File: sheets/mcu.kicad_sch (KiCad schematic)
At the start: 10 parts, among them U1 STM32F072CBTx

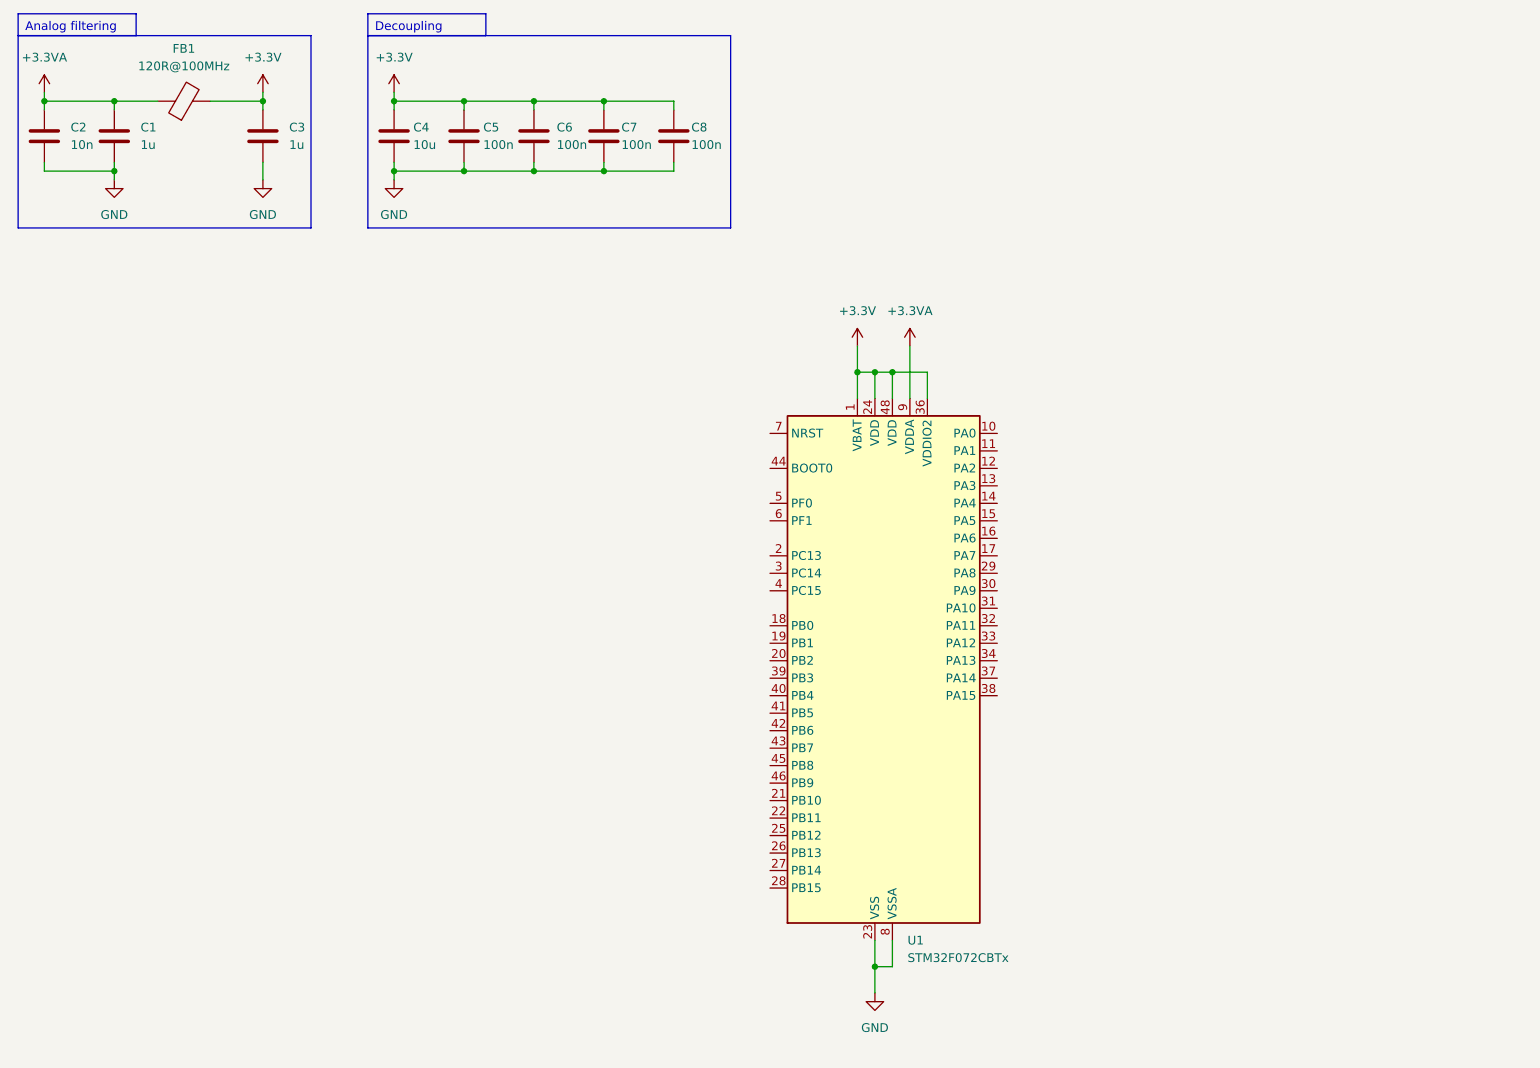
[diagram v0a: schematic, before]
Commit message: fsdfsdf
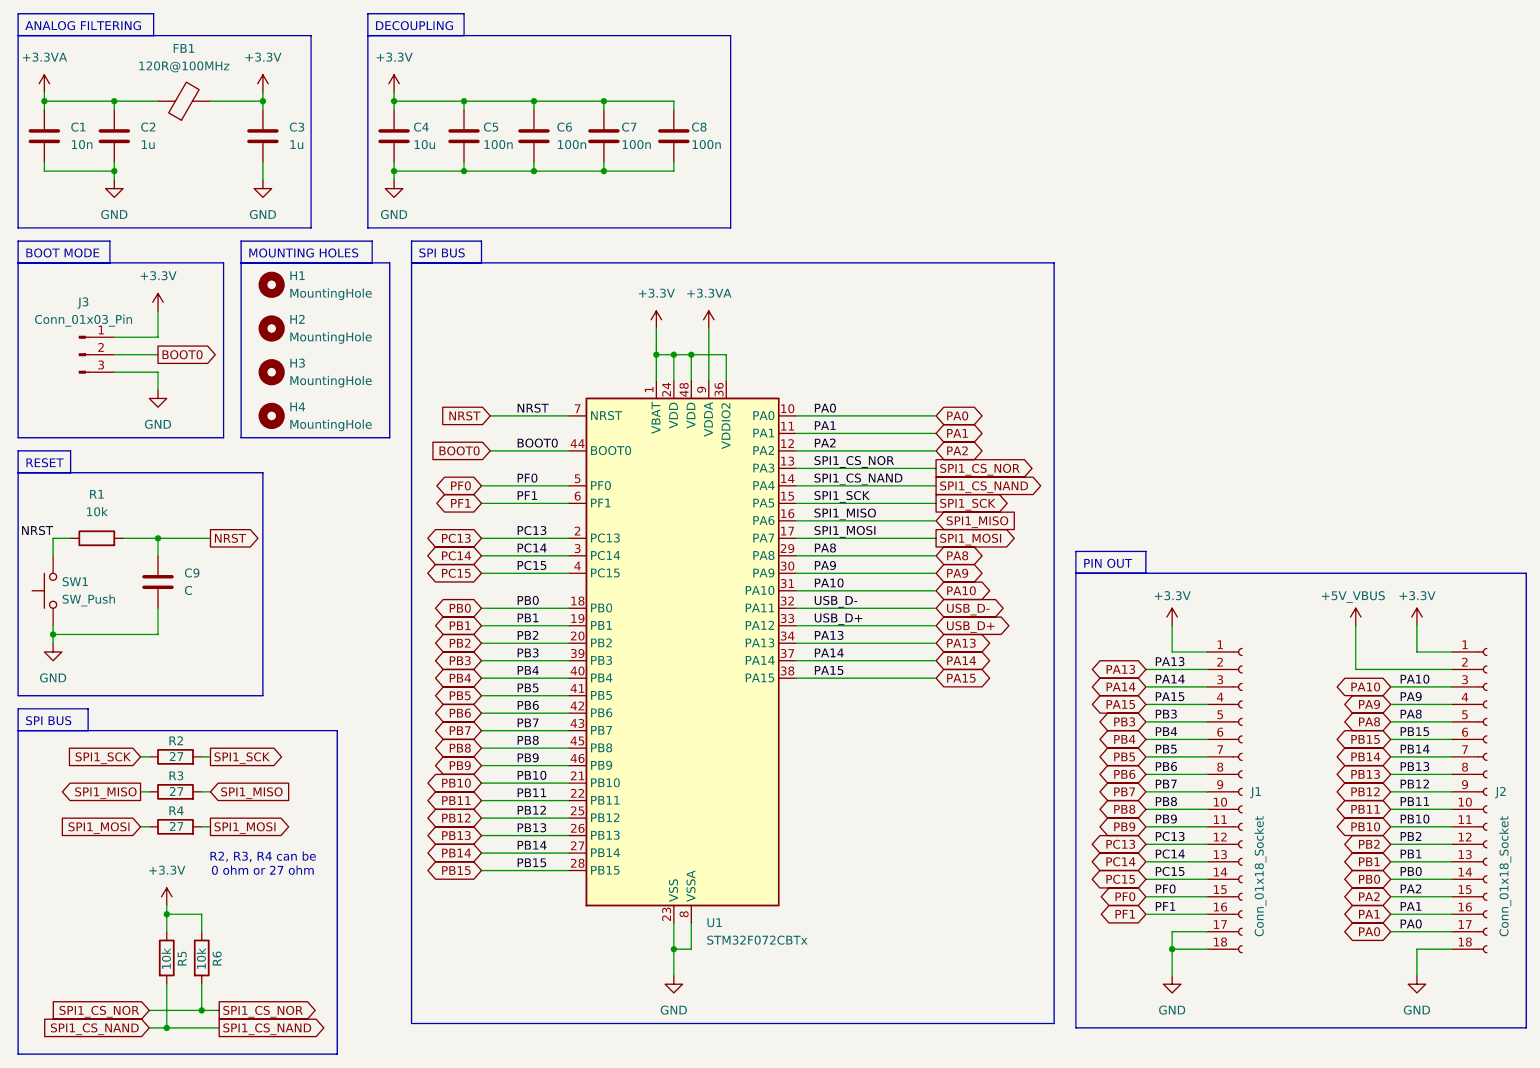
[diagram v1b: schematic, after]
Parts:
- added C9: C, Capacitor_SMD:C_0603_1608Metric, symbol Device:C
- added H1, H2, H3, H4: MountingHole, MountingHole:MountingHole_2.2mm_M2_DIN965, symbol Mechanical:MountingHole
- added J1, J2: Conn_01x18_Socket, Connector_PinSocket_2.54mm:PinSocket_1x18_P2.54mm_Vertical, symbol Connector:Conn_01x18_Socket
- added J3: Conn_01x03_Pin, Connector_PinHeader_2.54mm:PinHeader_1x03_P2.54mm_Vertical, symbol Connector:Conn_01x03_Pin
- added R1, R5, R6: 10k, Resistor_SMD:R_0603_1608Metric, symbol Device:R
- added R2, R3, R4: 27, Resistor_SMD:R_0603_1608Metric, symbol Device:R
- added SW1: SW_Push, Button_Switch_SMD:SW_Push_SPST_NO_Alps_SKRK, symbol Switch:SW_Push
- FB1: footprint (none) -> Resistor_SMD:R_0603_1608Metric
- renumbered C2 to C1, C1 to C2
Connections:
- net +3.3V: now also J1.1 (Pin_1), J2.1 (Pin_1), J3.1 (Pin_1), R5.1, R6.1
- net GND: now also C9.2, J1.17 (Pin_17), J1.18 (Pin_18), J2.18 (Pin_18), J3.3 (Pin_3), SW1.1
- net PA0: now reaches U1.10 (PA0)
- net PA0: now also J2.17 (Pin_17)
- net PA1: now reaches U1.11 (PA1)
- net PA1: now also J2.16 (Pin_16)
- net PA2: now reaches U1.12 (PA2)
- net PA2: now also J2.15 (Pin_15)
- net SPI1_CS_NOR: now reaches U1.13 (PA3)
- net SPI1_CS_NOR: now also R6.2
- net SPI1_CS_NAND: now reaches U1.14 (PA4)
- net SPI1_CS_NAND: now also R5.2
- net SPI1_SCK: now reaches U1.15 (PA5)
- net SPI1_SCK: now also R2.1, R2.2
- net SPI1_MISO: now reaches U1.16 (PA6)
- net SPI1_MISO: now also R3.1, R3.2
- net SPI1_MOSI: now reaches U1.17 (PA7)
- net SPI1_MOSI: now also R4.1, R4.2
- net PB0: now reaches U1.18 (PB0)
- net PB0: now also J2.14 (Pin_14)
- net PB1: now reaches U1.19 (PB1)
- net PB1: now also J2.13 (Pin_13)
- net PC13: now reaches U1.2 (PC13)
- net PC13: now also J1.12 (Pin_12)
- net PB2: now reaches U1.20 (PB2)
- net PB2: now also J2.12 (Pin_12)
- net PB10: now reaches U1.21 (PB10)
- net PB10: now also J2.11 (Pin_11)
- net PB11: now reaches U1.22 (PB11)
- net PB11: now also J2.10 (Pin_10)
- net PB12: now reaches U1.25 (PB12)
- net PB12: now also J2.9 (Pin_9)
- net PB13: now reaches U1.26 (PB13)
- net PB13: now also J2.8 (Pin_8)
- net PB14: now reaches U1.27 (PB14)
- net PB14: now also J2.7 (Pin_7)
- net PB15: now reaches U1.28 (PB15)
- net PB15: now also J2.6 (Pin_6)
- net PA8: now reaches U1.29 (PA8)
- net PA8: now also J2.5 (Pin_5)
- net PC14: now reaches U1.3 (PC14)
- net PC14: now also J1.13 (Pin_13)
- net PA9: now reaches U1.30 (PA9)
- net PA9: now also J2.4 (Pin_4)
- net PA10: now reaches U1.31 (PA10)
- net PA10: now also J2.3 (Pin_3)
- net USB_D-: now reaches U1.32 (PA11)
- net USB_D+: now reaches U1.33 (PA12)
- net PA13: now reaches U1.34 (PA13)
- net PA13: now also J1.2 (Pin_2)
- net PA14: now reaches U1.37 (PA14)
- net PA14: now also J1.3 (Pin_3)
- net PA15: now reaches U1.38 (PA15)
- net PA15: now also J1.4 (Pin_4)
- net PB3: now reaches U1.39 (PB3)
- net PB3: now also J1.5 (Pin_5)
- net PC15: now reaches U1.4 (PC15)
- net PC15: now also J1.14 (Pin_14)
- net PB4: now reaches U1.40 (PB4)
- net PB4: now also J1.6 (Pin_6)
- net PB5: now reaches U1.41 (PB5)
- net PB5: now also J1.7 (Pin_7)
- net PB6: now reaches U1.42 (PB6)
- net PB6: now also J1.8 (Pin_8)
- net PB7: now reaches U1.43 (PB7)
- net PB7: now also J1.9 (Pin_9)
- net BOOT0: now reaches U1.44 (BOOT0)
- net BOOT0: now also J3.2 (Pin_2)
- net PB8: now reaches U1.45 (PB8)
- net PB8: now also J1.10 (Pin_10)
- net PB9: now reaches U1.46 (PB9)
- net PB9: now also J1.11 (Pin_11)
- net PF0: now reaches U1.5 (PF0)
- net PF0: now also J1.15 (Pin_15)
- net PF1: now reaches U1.6 (PF1)
- net PF1: now also J1.16 (Pin_16)
- net NRST: now reaches U1.7 (NRST)
- net NRST: now also C9.1, R1.1, R1.2, SW1.2
- new net +5V_VBUS: J2.2 (Pin_2)
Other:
- note added: "R2, R3, R4 can be 0 ohm or 27 ohm"
- moved on the sheet: U1
